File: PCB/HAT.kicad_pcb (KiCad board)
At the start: 2 copper layers, 99.3 x 98.9 mm, 103 parts, among them J1 Conn_01x02_Pin, J10 Conn_01x24_Socket, J11 Conn_01x24_Pin, J12 Conn_01x02_Pin, J13 Conn_01x02_Pin, J14 Conn_01x02_Pin, J15 Conn_01x02_Pin, J2 Conn_01x02_Pin, J3 Conn_01x01_Pin, J4 Conn_01x02_Pin, J5 Conn_01x10_Pin, J6 MICROXNJ, J7 Conn_01x01_Pin, J8 Conn_01x24_Pin, J9 Conn_01x24_Socket, Q1 AO3401A, Q2 LBSS84LT1G, Q3 LBSS84LT1G, Q4 BSS138, Q5 BSS138, Q6 BSS138, Q7 BSS138, Q8 LM317AG-TN3-R, U1 TP4056, U2 XC6206P, U3 MCP6002-xMC, U4 VL6180, U6 CAT24C256, U7 CH340C, Y1 C252310

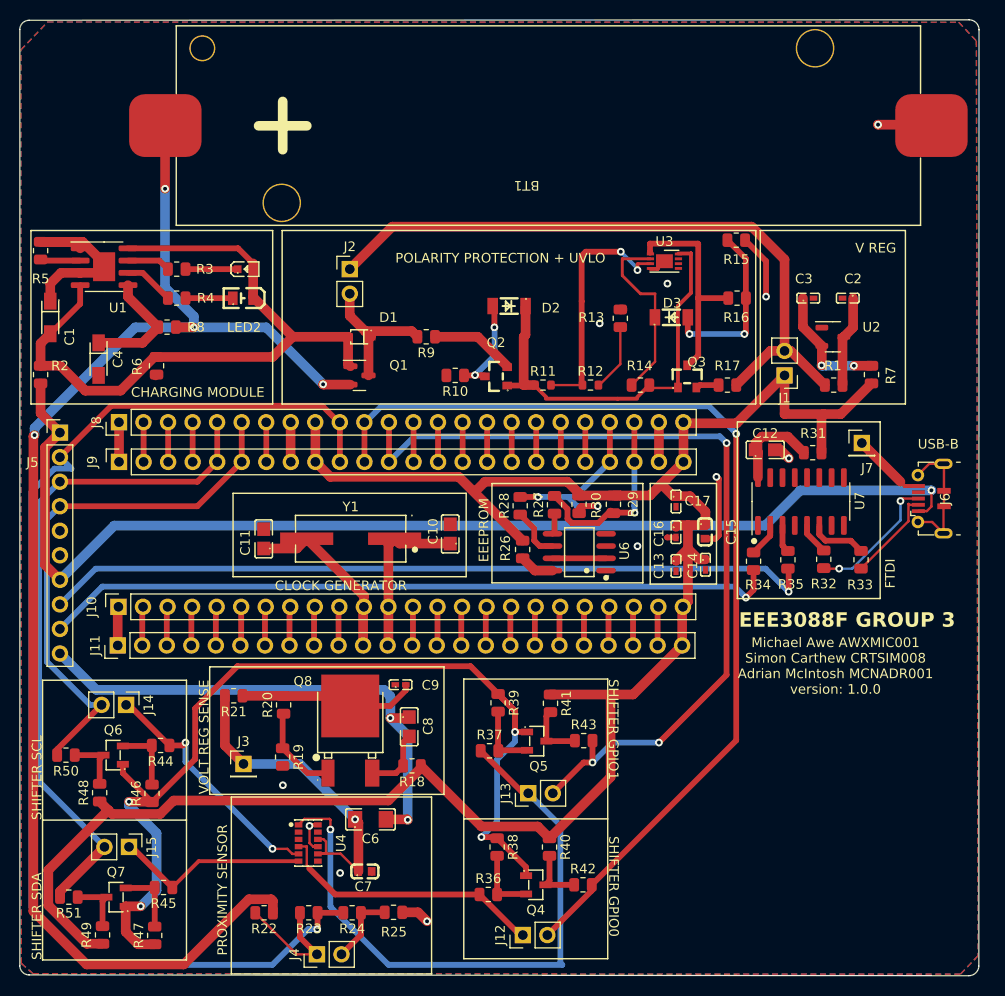
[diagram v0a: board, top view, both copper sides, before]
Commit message: simon changes
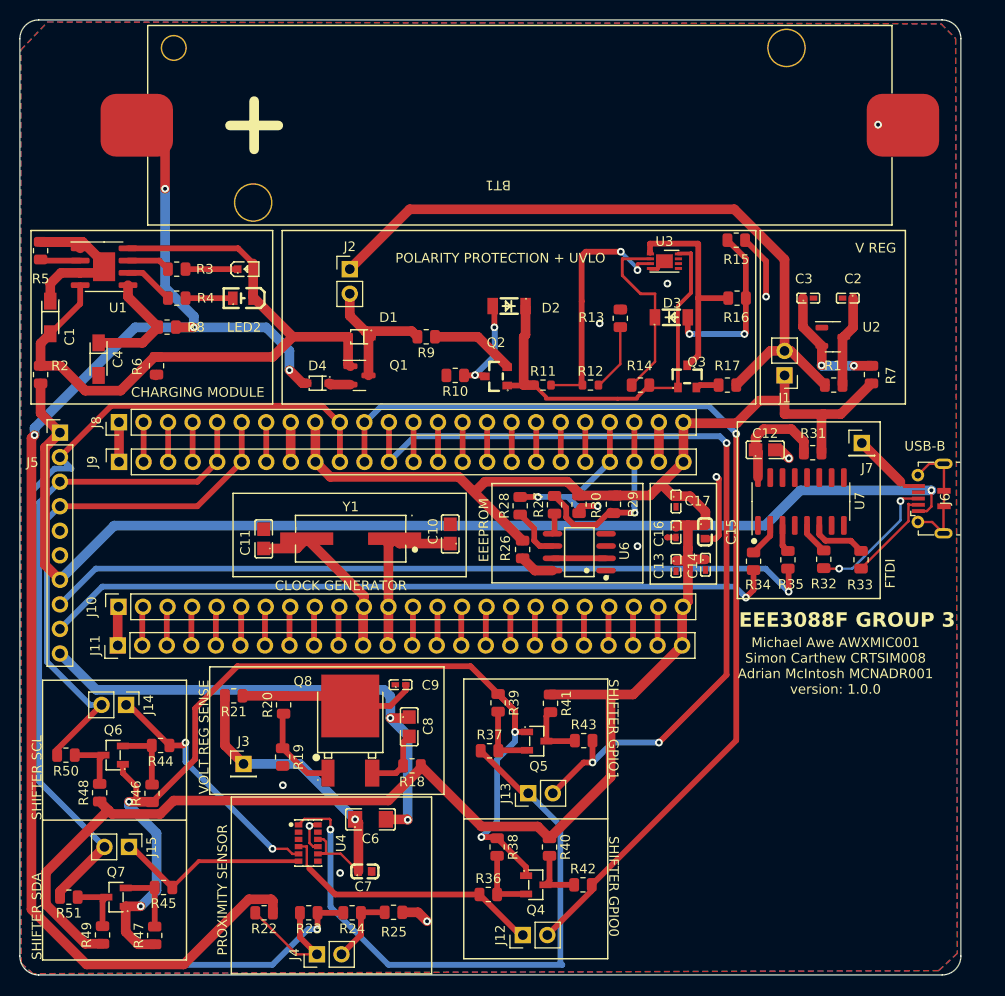
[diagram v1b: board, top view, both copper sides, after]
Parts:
- added D4: D_Schottky, JLC_Diodes:SOD-323_L1.8-W1.3-LS2.5-RD, F.Cu at (127.3, 84.5)
- moved BT1 2.96 mm to (148.2, 57.2)
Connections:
- Q1 pad 2: /Power Module/V_BAT+ -> Net-(D4-K)
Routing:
- net /Power Module/V_BAT+: track 144.7 -> 141.5 mm
- net Net-(D4-K): track 0.00 -> 2.25 mm
- net /MicroController_Interfacing/3V3: track 220.9 -> 219.2 mm
- net Net-(U7-VCC): track 9.65 -> 11.3 mm
- net /Power Module/UVLO_3V3: track 69.8 -> 71.3 mm
- net /Sensor Module/Logic Level Shifting/2V8: track 103.6 -> 102.9 mm
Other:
- board size 99.3 x 98.9 mm -> 97.4 x 98.8 mm

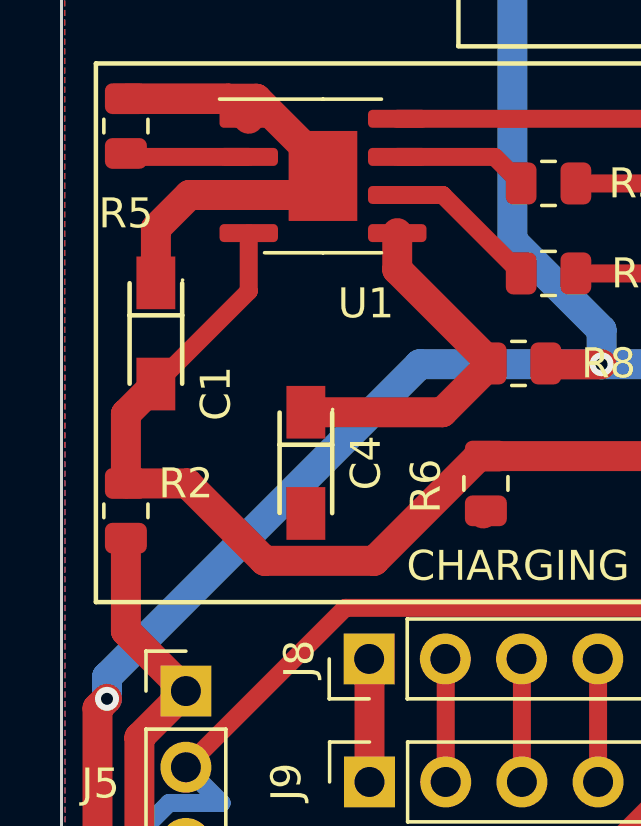
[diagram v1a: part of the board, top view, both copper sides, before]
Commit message: final pcb and chematic changes
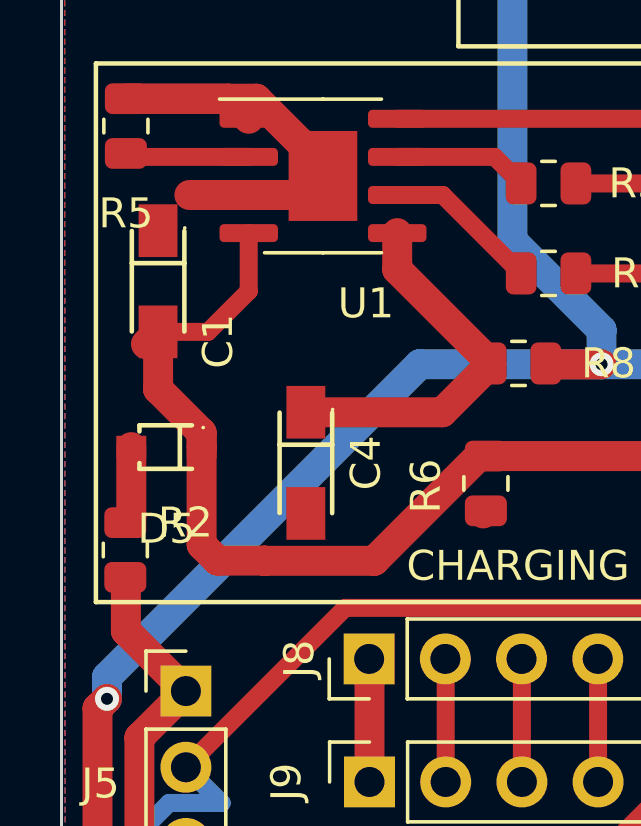
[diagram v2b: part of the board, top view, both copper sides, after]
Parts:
- added D5: D_Schottky, JLC_Diodes:SOD-323_L1.8-W1.3-LS2.5-RD, F.Cu at (99.9, 81.4)
- moved C1 1.74 mm to (99.7, 75.9)
- moved R2 1.31 mm to (98.6, 84.9)
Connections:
- R2 pad 2: Net-(D1-A) -> Net-(D5-A)
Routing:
- net GND: track 127.9 -> 124.5 mm
- net Net-(D5-A): track 0.00 -> 2.60 mm
- net /MicroController_Interfacing/USB 5V: track 119.7 -> 118.4 mm
